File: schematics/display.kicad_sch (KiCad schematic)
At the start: 56 parts, among them Q11 2N3906, Q9 2N3906, U14 74AC138, U15 74HC245, U16 74HC245, U17 74HC245, U18 74HC245, U19 74HC4511, U20 74HC4511, U25 RED, U26 RED, U27 RED, U28 RED, U29 RED, U30 RED, U31 RED, U32 RED, U33 RED

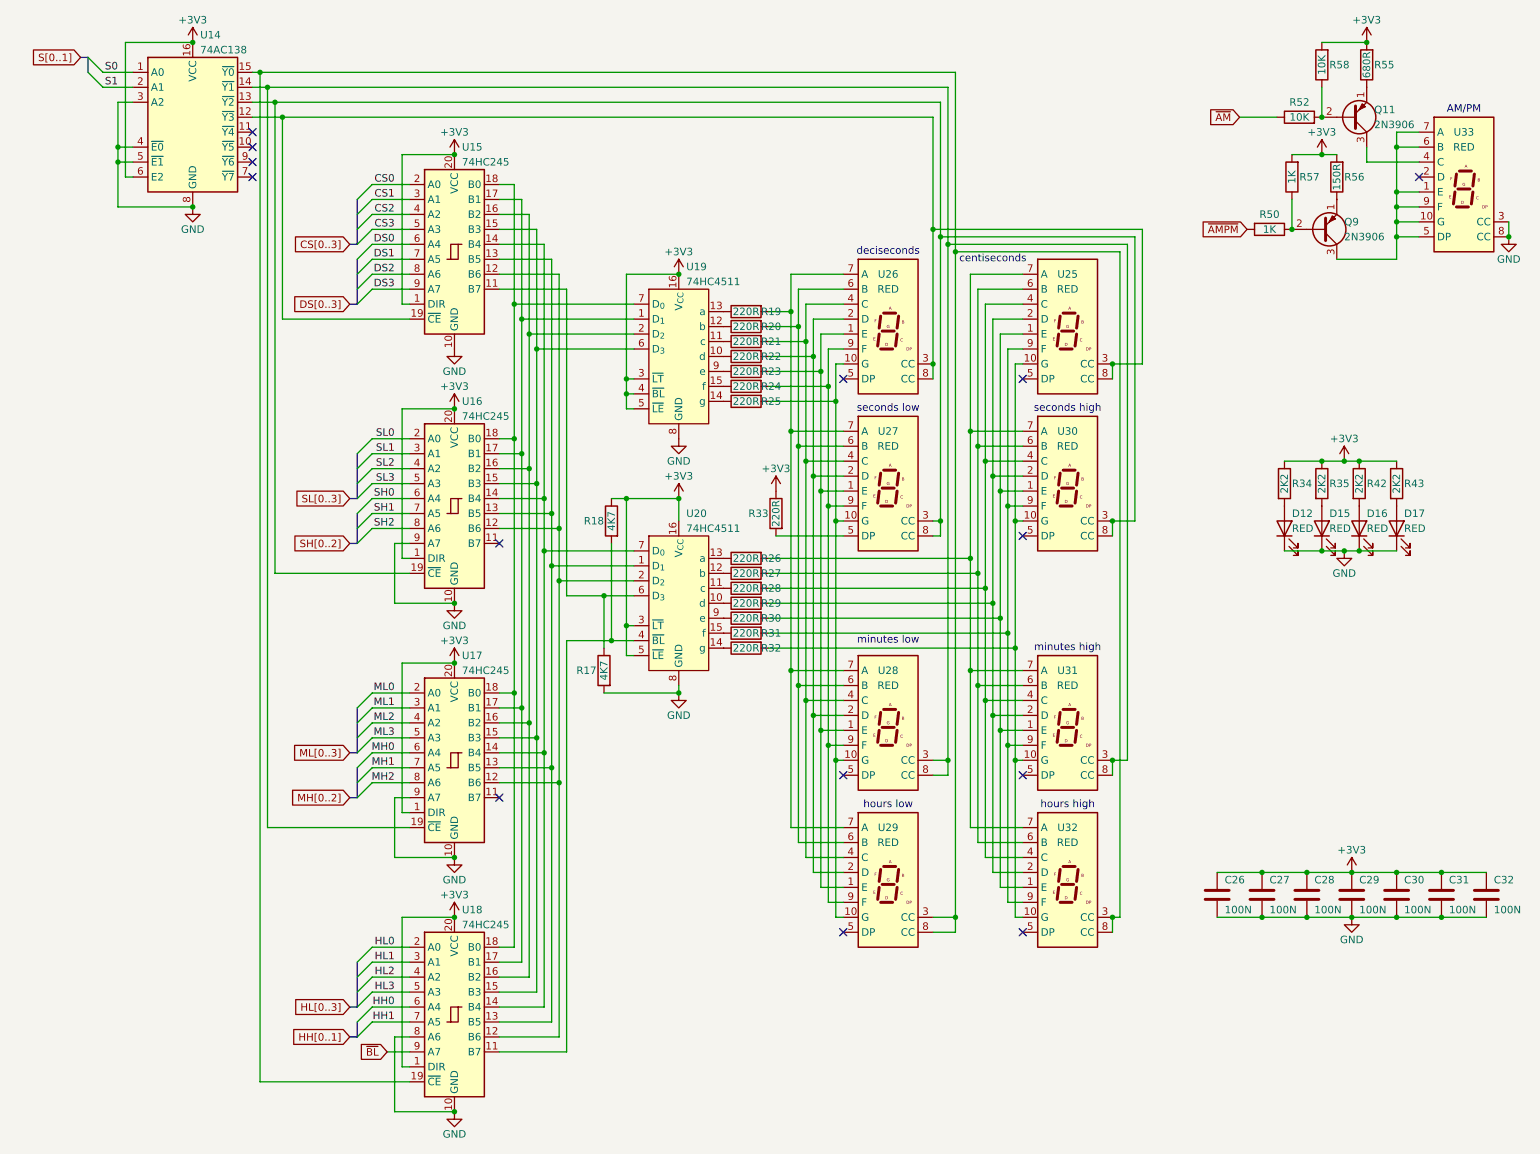
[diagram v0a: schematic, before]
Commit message: started a second version
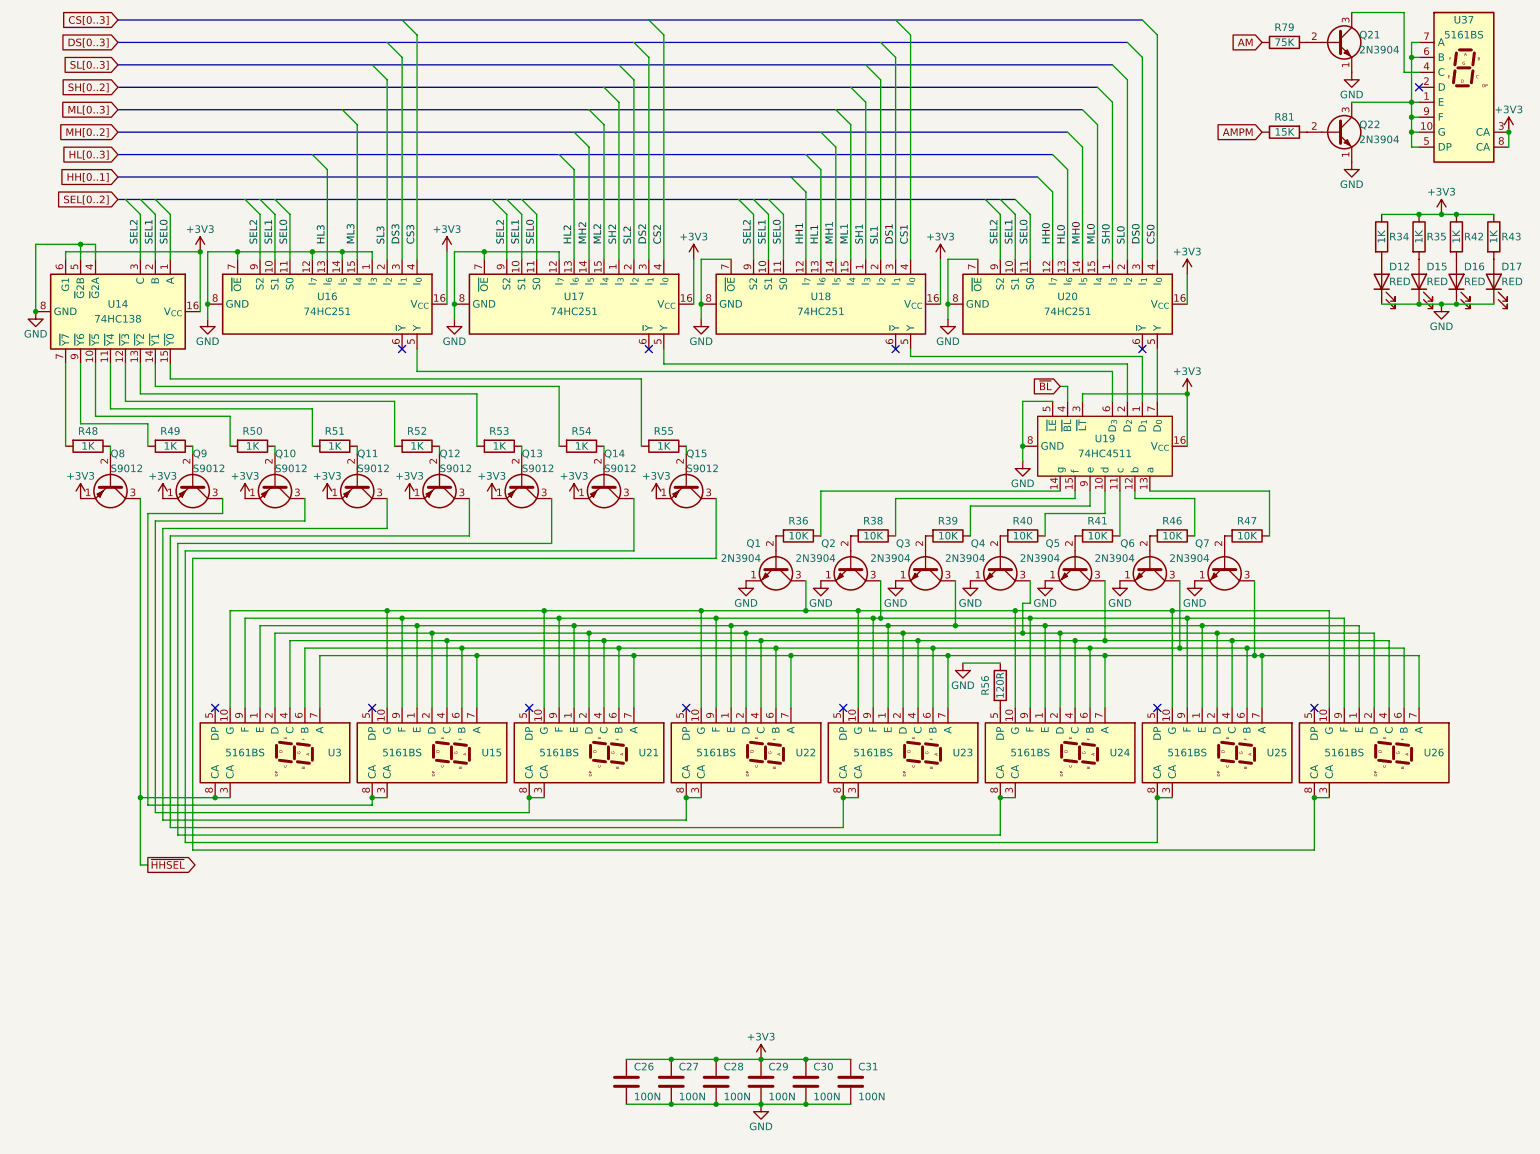
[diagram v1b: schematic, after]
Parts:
- removed C32: 100N, Package_SO:SOIC-8_3.9x4.9mm_P1.27mm, symbol Device:C
- removed Q11, Q9: 2N3906, Package_TO_SOT_THT:TO-92_Inline, symbol Transistor_BJT:2N3906
- removed R17, R18: 4K7, symbol Device:R
- removed R19, R20, R21, R22, R23, R24, R25, R26, R27, R28, R29, R30, R31, R32, R33: 220R, symbol Device:R
- removed R57: 1K, symbol Device:R
- removed R58: 10K, symbol Device:R
- removed U15, U16, U17, U18: 74HC245, Package_SO:SOIC-16W_7.5x10.3mm_P1.27mm, symbol 74xx:74HC245
- removed U20: 74HC4511, symbol bvclock:74HC4511
- removed U25, U26, U27, U28, U29, U30, U31, U32, U33: RED, Display_7Segment:HDSP-A151, symbol Display_Character:HDSP-A153
- added Q1, Q2, Q21, Q22, Q3, Q4, Q5, Q6, Q7: 2N3904, Package_TO_SOT_THT:TO-92_Inline, symbol Transistor_BJT:2N3904
- added Q10, Q11, Q12, Q13, Q14, Q15, Q8, Q9: S9012, Package_TO_SOT_THT:TO-92_Inline, symbol Transistor_BJT:Q_PNP_EBC
- added R36, R38, R39, R40, R41, R46, R47: 10K, symbol Device:R
- added R48, R49, R51, R53, R54: 1K, symbol Device:R
- added R79: 75K, symbol Device:R
- added R81: 15K, symbol Device:R
- added U15, U21, U22, U23, U24, U25, U26, U3, U37: 5161BS, Display_7Segment:KCSC02-105, symbol Display_Character:KCSA02-105
- added U16, U17, U18, U20: 74HC251, Package_DIP:DIP-28_W15.24mm, symbol 74xx:74LS251
- R34, R35, R42, R43: value 2K2 -> 1K
- R52: value 10K -> 1K
- R55: value 680R -> 1K
- R56: value 150R -> 120R
- U14: value 74AC138 -> 74HC138
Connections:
- net ~{AMPM} is gone; now on an unnamed net: R50.2
- net +3V3: now also Q10.1 (E), Q11.1 (E), Q12.1 (E), Q13.1 (E), Q14.1 (E), Q15.1 (E), Q8.1 (E), Q9.1 (E), U16.16 (V_{CC}), U17.16 (V_{CC}), U18.16 (V_{CC}), U20.16 (V_{CC}), U37.3 (CA), U37.8 (CA); no longer R55.2, R56.2, U19.4 (~{BL}), U19.5 (~{LE})
- net CS0: now also U20.4 (I_{0})
- net CS1: now also U18.4 (I_{0})
- net CS2: now also U17.4 (I_{0})
- net CS3: now also U16.4 (I_{0})
- net DS0: now also U20.3 (I_{1})
- net DS1: now also U18.3 (I_{1})
- net DS2: now also U17.3 (I_{1})
- net DS3: now also U16.3 (I_{1})
- net GND: now also R56.1, U19.5 (~{LE}), Q1.1 (E), Q2.1 (E), Q21.1 (E), Q22.1 (E), Q3.1 (E), Q4.1 (E), Q5.1 (E), Q6.1 (E), Q7.1 (E), U16.1 (I_{3}), U16.12 (I_{7}), U16.14 (I_{5}), U16.7 (~{OE}), U16.8 (GND), U17.12 (I_{7}), U17.7 (~{OE}), U17.8 (GND), U18.7 (~{OE}), U18.8 (GND), U20.7 (~{OE}), U20.8 (GND); no longer U14.3 (A2)
- net HH0: now also U20.12 (I_{7})
- net HH1: now also U18.12 (I_{7})
- net HL0: now also U20.13 (I_{6})
- net HL1: now also U18.13 (I_{6})
- net HL2: now also U17.13 (I_{6})
- net HL3: now also U16.13 (I_{6})
- net MH0: now also U20.14 (I_{5})
- net MH1: now also U18.14 (I_{5})
- net MH2: now also U17.14 (I_{5})
- net ML0: now also U20.15 (I_{4})
- net ML1: now also U18.15 (I_{4})
- net ML2: now also U17.15 (I_{4})
- net ML3: now also U16.15 (I_{4})
- net SH0: now also U20.1 (I_{3})
- net SH1: now also U18.1 (I_{3})
- net SH2: now also U17.1 (I_{3})
- net SL0: now also U20.2 (I_{2})
- net SL1: now also U18.2 (I_{2})
- net SL2: now also U17.2 (I_{2})
- net SL3: now also U16.2 (I_{2})
- net ~{BL}: now also U19.4 (~{BL})
- net at U19.12 (b): now also R46.1
- net at R52.2: now also U14.12 (~{Y3})
- net at U19.10 (d): now also R40.1
- net at U19.6 (D_{3}): now also U16.5 (Y)
- net at U19.2 (D_{2}): now also U17.5 (Y)
- net at U19.1 (D_{1}): now also U18.5 (Y)
- net at U19.7 (D_{0}): now also U20.5 (Y)
- net at U19.13 (a): now also R47.1
- net at U19.11 (c): now also R41.1
- net at U14.14 (~{Y1}): now also R54.2
- net at U19.15 (f): now also R38.1
- net at U14.15 (~{Y0}): now also R55.2
- net at R50.1: now also Q10.2 (B)
- net at R55.1: now also Q15.2 (B)
- net at U19.9 (e): now also R39.1
- net at U14.13 (~{Y2}): now also R53.2
- net at U19.14 (g): now also R36.1
- net at U14.11 (~{Y4}): now also R51.2
- net at U14.7 (~{Y7}): now also R48.2
- net at U14.9 (~{Y6}): now also R49.2
- net S0 renamed SEL0
- net SEL0: now also U16.11 (S0), U17.11 (S0), U18.11 (S0), U20.11 (S0)
- net S1 renamed SEL1
- net SEL1: now also U16.10 (S1), U17.10 (S1), U18.10 (S1), U20.10 (S1)
- net ~{AM}: no longer names the net of R52.1
- net ~{AM}: now also Q12.2 (B)
- new net: Q22.2 (B), R81.2
- new net: Q22.3 (C), U37.1 (E), U37.10 (G), U37.5 (DP), U37.6 (B), U37.7 (A), U37.9 (F)
- new net: Q6.2 (B), R46.2
- new net: Q6.3 (C), U15.6 (B), U21.6 (B), U22.6 (B), U23.6 (B), U24.6 (B), U25.6 (B), U26.6 (B), U3.6 (B)
- new net: Q3.3 (C), U15.1 (E), U21.1 (E), U22.1 (E), U23.1 (E), U24.1 (E), U25.1 (E), U26.1 (E), U3.1 (E)
- new net: Q1.3 (C), U15.10 (G), U21.10 (G), U22.10 (G), U23.10 (G), U24.10 (G), U25.10 (G), U26.10 (G), U3.10 (G)
- new net: Q4.3 (C), U15.2 (D), U21.2 (D), U22.2 (D), U23.2 (D), U24.2 (D), U25.2 (D), U26.2 (D), U3.2 (D)
- new net: Q13.3 (C), U24.3 (CA), U24.8 (CA)
- new net: Q5.3 (C), U15.4 (C), U21.4 (C), U22.4 (C), U23.4 (C), U24.4 (C), U25.4 (C), U26.4 (C), U3.4 (C)
- new net: R56.2, U24.5 (DP)
- new net: Q7.3 (C), U15.7 (A), U21.7 (A), U22.7 (A), U23.7 (A), U24.7 (A), U25.7 (A), U26.7 (A), U3.7 (A)
- new net: Q2.3 (C), U15.9 (F), U21.9 (F), U22.9 (F), U23.9 (F), U24.9 (F), U25.9 (F), U26.9 (F), U3.9 (F)
- new net: Q15.3 (C), U26.3 (CA), U26.8 (CA)
- new net: Q4.2 (B), R40.2
- new net: Q3.2 (B), R39.2
- new net: Q7.2 (B), R47.2
- new net: Q1.2 (B), R36.2
- new net: Q8.2 (B), R48.1
- new net: Q11.3 (C), U22.3 (CA), U22.8 (CA)
- new net: Q12.3 (C), U23.3 (CA), U23.8 (CA)
- new net: Q2.2 (B), R38.2
- new net: Q11.2 (B), R51.1
- new net: Q21.2 (B), R79.2
- new net: Q10.3 (C), U21.3 (CA), U21.8 (CA)
- new net: Q13.2 (B), R53.1
- new net: Q14.2 (B), R54.1
- new net: Q14.3 (C), U25.3 (CA), U25.8 (CA)
- new net: Q9.2 (B), R49.1
- new net: Q9.3 (C), U15.3 (CA), U15.8 (CA)
- new net: Q5.2 (B), R41.2
- new net: Q21.3 (C), U37.4 (C)
- new net AM: R79.1
- new net AMPM: R81.1
- new net SEL2: U14.3 (C), U16.9 (S2), U17.9 (S2), U18.9 (S2), U20.9 (S2)
- new net ~{HHSEL}: Q8.3 (C), U3.3 (CA), U3.8 (CA)
- no-connect marks 14 -> 12
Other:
- note removed: "AM/PM"
- note removed: "centiseconds"
- note removed: "deciseconds"
- note removed: "hours high"
- note removed: "hours low"
- note removed: "minutes high"
- note removed: "minutes low"
- note removed: "seconds high"
- note removed: "seconds low"
- moved on the sheet: C26, C27, C28, C29, C30, C31, D12, D15, D16, D17, R34, R35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
